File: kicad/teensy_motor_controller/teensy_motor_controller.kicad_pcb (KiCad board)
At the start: 2 copper layers, 57.4 x 61.4 mm, 12 parts, among them J1 Conn_01x11, U1 Teensy4.0

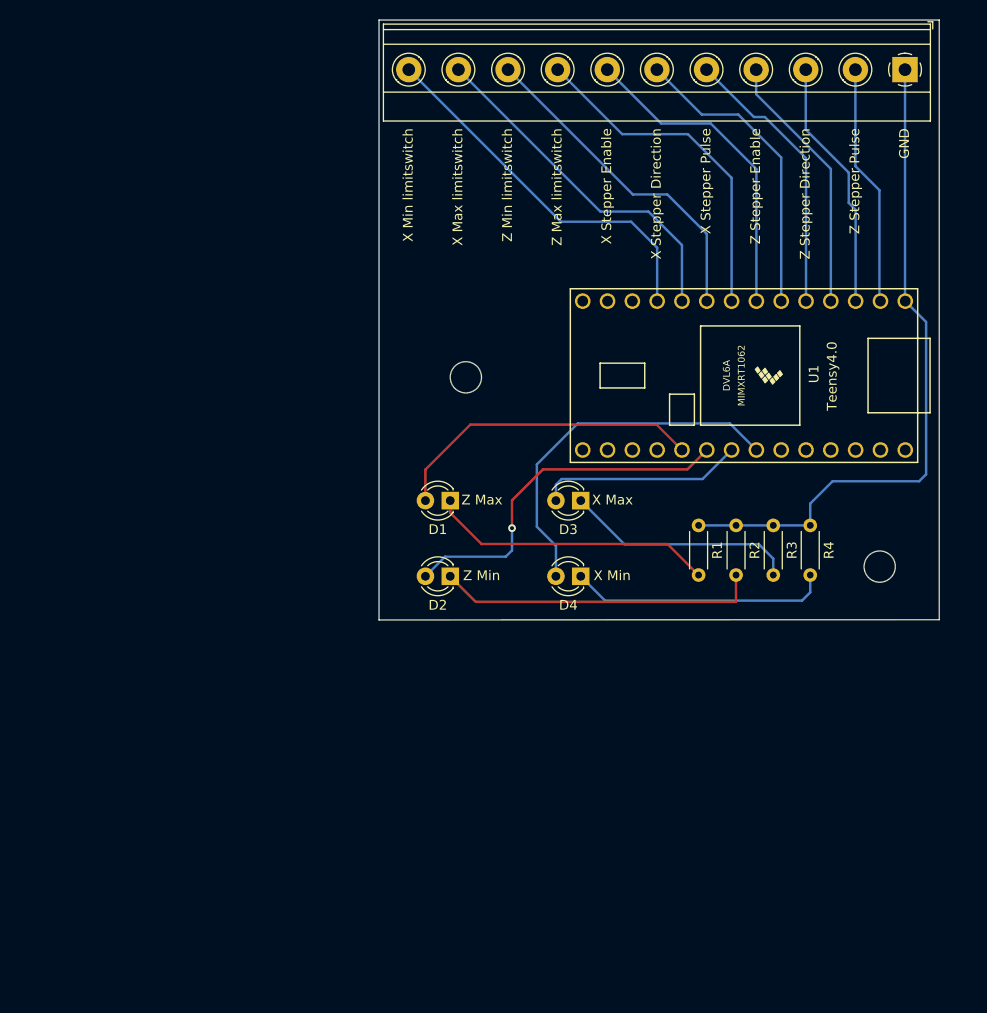
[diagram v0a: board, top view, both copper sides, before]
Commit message: New functionality
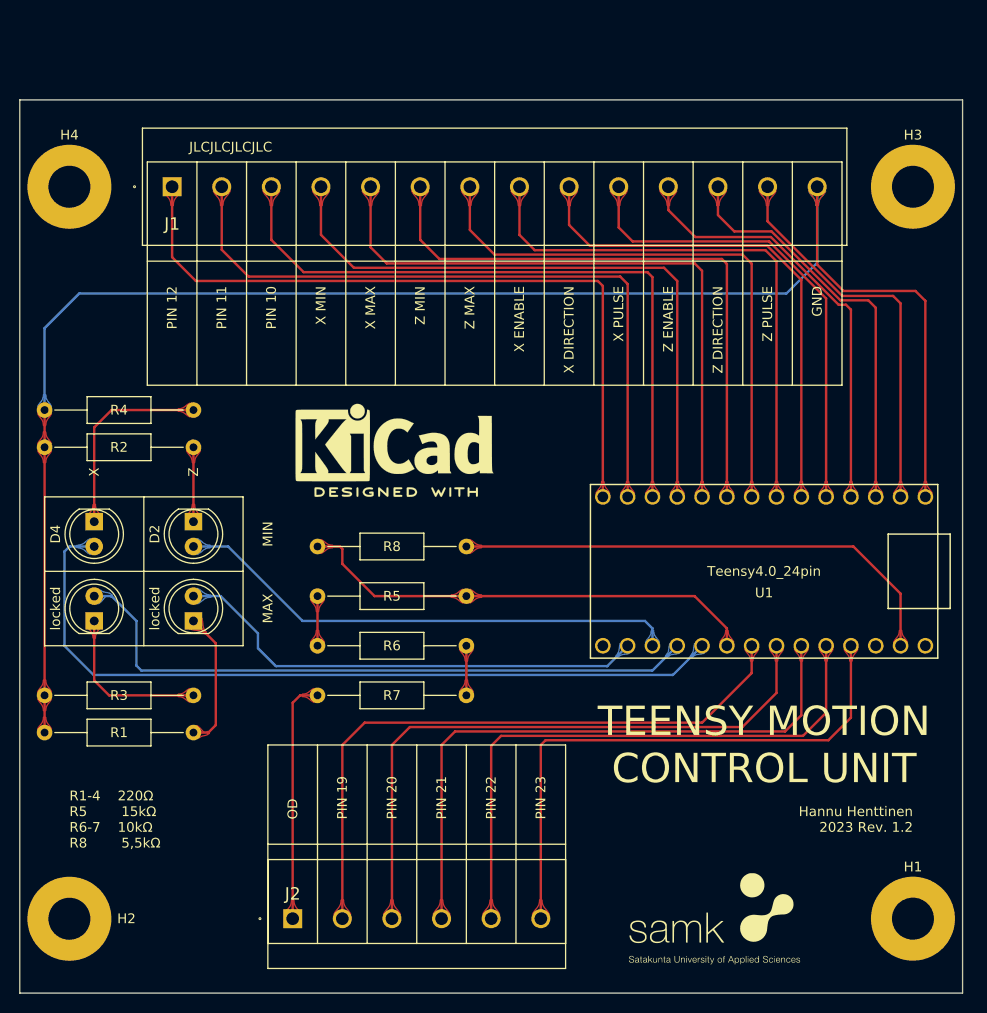
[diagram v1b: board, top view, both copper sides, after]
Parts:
- removed D1, D3: LED, LED_THT:LED_D3.0mm
- removed the REF** at (144.7, 76.7)
- removed the REF** at (187.1, 96.0)
- added G***: LOGO, art:samk_logo, F.Cu at (170.2, 132.1)
- added H1: MountingHole, MountingHole:MountingHole_4.3mm_M4_Pad, F.Cu at (190.5, 132.1)
- added H2: MountingHole, MountingHole:MountingHole_4.3mm_M4_Pad, F.Cu at (104.1, 132.1)
- added H3: MountingHole, MountingHole:MountingHole_4.3mm_M4_Pad, F.Cu at (190.5, 57.1)
- added H4: MountingHole, MountingHole:MountingHole_4.3mm_M4_Pad, F.Cu at (104.1, 57.1)
- added J2: 1730162, SamacSys_Parts:1730162, F.Cu at (127.0, 132.1)
- added R5: R15k, Resistor_THT:R_Axial_DIN0207_L6.3mm_D2.5mm_P15.24mm_Horizontal, F.Cu at (129.5, 99.1)
- added R6: R10k, Resistor_THT:R_Axial_DIN0207_L6.3mm_D2.5mm_P15.24mm_Horizontal, F.Cu at (129.5, 104.1)
- added R7: R10k, Resistor_THT:R_Axial_DIN0207_L6.3mm_D2.5mm_P15.24mm_Horizontal, F.Cu at (144.8, 109.2)
- added R8: R5,5k, Resistor_THT:R_Axial_DIN0207_L6.3mm_D2.5mm_P15.24mm_Horizontal, F.Cu at (144.8, 94.0)
- added REF**: KiCad-Logo2_8mm_SilkScreen, Symbol:KiCad-Logo2_8mm_SilkScreen, F.Cu at (137.4, 83.3)
- added locked: LED, LED_THT:LED_D5.0mm, F.Cu at (106.7, 101.6)
- added locked: LED, LED_THT:LED_D5.0mm, F.Cu at (116.8, 101.6)
- D2, D4: footprint LED_THT:LED_D3.0mm -> LED_THT:LED_D5.0mm
- J1: value Conn_01x11 -> 1869334; footprint TerminalBlock_Phoenix:TerminalBlock_Phoenix_MKDS-1,5-11-5.08_1x11_P5.08mm_Horizontal -> SamacSys_Parts:1869334
- R1, R2, R3, R4: footprint Resistor_THT:R_Axial_DIN0204_L3.6mm_D1.6mm_P5.08mm_Horizontal -> Resistor_THT:R_Axial_DIN0207_L6.3mm_D2.5mm_P15.24mm_Horizontal
- U1: value Teensy4.0 -> Teensy4.0_24pin; footprint teensy:Teensy40_side_pins -> teensy:Teensy40_24pin
- moved R4 79.3 mm to (101.6, 80.0), turned to 0 degrees
- moved R3 76.6 mm to (101.6, 109.2), turned to 0 degrees
- moved J1 76.0 mm to (114.7, 57.1), turned to 0 degrees
- moved R2 71.2 mm to (101.6, 83.8), turned to 0 degrees
- moved R1 70.2 mm to (101.6, 113.0), turned to 0 degrees
- moved D4 50.1 mm to (106.7, 91.4), turned to -90 degrees
- moved D2 26.9 mm to (116.8, 91.4), turned to -90 degrees
- moved U1 20.1 mm to (175.3, 96.5)
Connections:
- J1 pad 10: /X_max_limit -> /X_stepper_pulse
- J1 pad 11: /X_min_limit -> /Z_stepper_enable
- J1 pad 2: /Z_stepper_pulse -> Net-(J1-Pad2)
- J1 pad 3: /Z_stepper_direction -> Net-(J1-Pad3)
- J1 pad 4: /Z_stepper_enable -> /X_min_limit
- J1 pad 5: /X_stepper_pulse -> /X_max_limit
- J1 pad 6: /X_stepper_direction -> /Z_min_limit
- J1 pad 7: /X_stepper_enable -> /Z_max_limit
- J1 pad 8: /Z_max_limit -> /X_stepper_enable
- J1 pad 9: /Z_min_limit -> /X_stepper_direction
- R1 pad 1: Net-(J1-Pad1) -> Net-(J1-Pad14)
- R2 pad 1: Net-(J1-Pad1) -> Net-(J1-Pad14)
- R3 pad 1: Net-(J1-Pad1) -> Net-(J1-Pad14)
- R4 pad 1: Net-(J1-Pad1) -> Net-(J1-Pad14)
- U1 pad 1: Net-(J1-Pad1) -> /Z_stepper_direction
- U1 pad 10: /X_max_limit -> Net-(J1-Pad3)
- U1 pad 11: /X_min_limit -> Net-(J1-Pad2)
- U1 pad 12: (no net) -> Net-(J1-Pad1)
- U1 pad 13: (no net) -> unconnected-(U1-Pad13)
- U1 pad 14: (no net) -> /Z_max_led
- U1 pad 2: /Z_stepper_pulse -> /Z_stepper_enable
- U1 pad 20: (no net) -> Net-(J2-Pad3)
- U1 pad 21: (no net) -> Net-(J2-Pad4)
- U1 pad 22: (no net) -> Net-(J2-Pad5)
- U1 pad 23: (no net) -> Net-(J2-Pad6)
- U1 pad 3: /Z_stepper_direction -> /X_stepper_pulse
- U1 pad 4: /Z_stepper_enable -> /X_stepper_direction
- U1 pad 5: /X_stepper_pulse -> /X_stepper_enable
- U1 pad 6: /X_stepper_direction -> /Z_max_limit
- U1 pad 7: /X_stepper_enable -> /Z_min_limit
- U1 pad 8: /Z_max_limit -> /X_max_limit
- U1 pad 9: /Z_min_limit -> /X_min_limit
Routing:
- net Net-(J1-Pad14): track 0.00 -> 171.7 mm
- net Net-(J1-Pad2): track 0.00 -> 71.3 mm
- net Net-(J1-Pad3): track 0.00 -> 68.5 mm
- net Net-(J2-Pad2): track 0.00 -> 65.5 mm
- net Net-(J2-Pad3): track 0.00 -> 64.2 mm
- net Net-(J2-Pad4): track 0.00 -> 63.0 mm
- net Net-(J2-Pad5): track 0.00 -> 60.2 mm
- net Net-(J2-Pad6): track 0.00 -> 58.1 mm
- net Net-(R8-Pad1): track 0.00 -> 51.8 mm
- net Net-(R5-Pad2): track 0.00 -> 48.1 mm
- net /X_max_led: track 21.1 -> 66.6 mm
- net /X_min_led: track 37.6 -> 80.7 mm
- net /X_max_limit: track 36.1 -> 64.3 mm
- net /Z_min_limit: track 34.2 -> 61.7 mm
- net /X_min_limit: track 38.4 -> 65.5 mm
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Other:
- board size 57.4 x 61.4 mm -> 96.5 x 91.4 mm
- net class Default removed
- board text added: "Hannu Henttinen 2023 Rev. 1.2"
- board text added: "JLCJLCJLCJLC"
- board text added: "MAX"
- board text added: "MIN"
- board text added: "OD"
- board text added: "PIN 10"
- board text added: "PIN 11"
- board text added: "PIN 12"
- board text added: "PIN 19"
- board text added: "PIN 20"
- board text added: "PIN 21"
- board text added: "PIN 22"
- board text added: "PIN 23"
- board text added: "R1-4 220Ω R5 15kΩ R6-7 10kΩ R8 5,5kΩ"
- board text added: "TEENSY MOTION CONTROL UNIT"
- board text added: "X"
- board text added: "X DIRECTION"
- board text added: "X ENABLE"
- board text added: "X MAX"
- board text added: "X MIN"
- board text added: "X PULSE"
- board text added: "Z"
- board text added: "Z DIRECTION"
- board text added: "Z ENABLE"
- board text added: "Z MAX"
- board text added: "Z MIN"
- board text added: "Z PULSE"
- board text removed: "Hannu Henttinen 2022 v1.1"
- board text removed: "X Max"
- board text removed: "X Max limitswitch"
- board text removed: "X Min"
- board text removed: "X Min limitswitch"
- board text removed: "X Stepper Direction"
- board text removed: "X Stepper Enable"
- board text removed: "X Stepper Pulse"
- board text removed: "Z Max"
- board text removed: "Z Max limitswitch"
- board text removed: "Z Min"
- board text removed: "Z Min limitswitch"
- board text removed: "Z Stepper Direction"
- board text removed: "Z Stepper Enable"
- board text removed: "Z Stepper Pulse"
